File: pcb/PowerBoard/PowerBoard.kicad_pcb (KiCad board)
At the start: 2 copper layers, 9 parts, among them P1 Motor battery, P2 CONN_01X06, P3 Arduino battery, SW1 OnOffDoubleSwitch

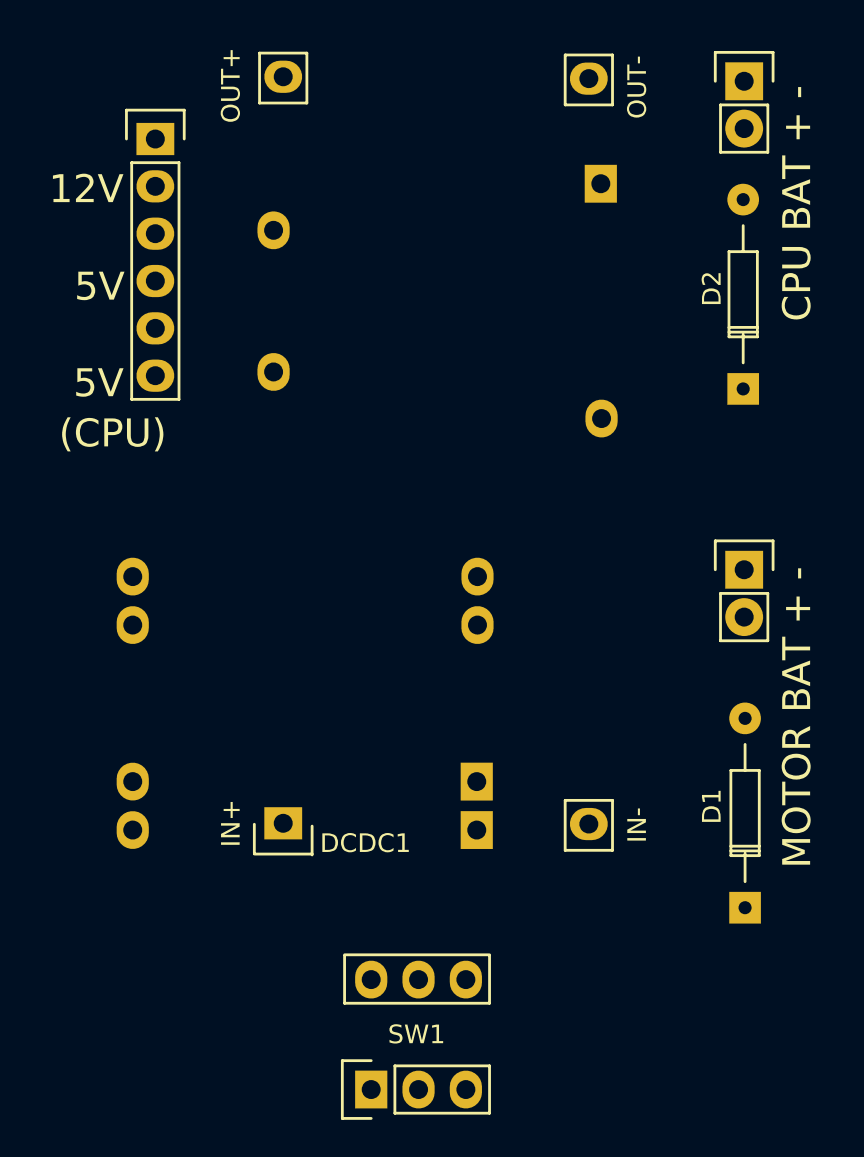
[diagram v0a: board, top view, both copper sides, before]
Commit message: power board ready
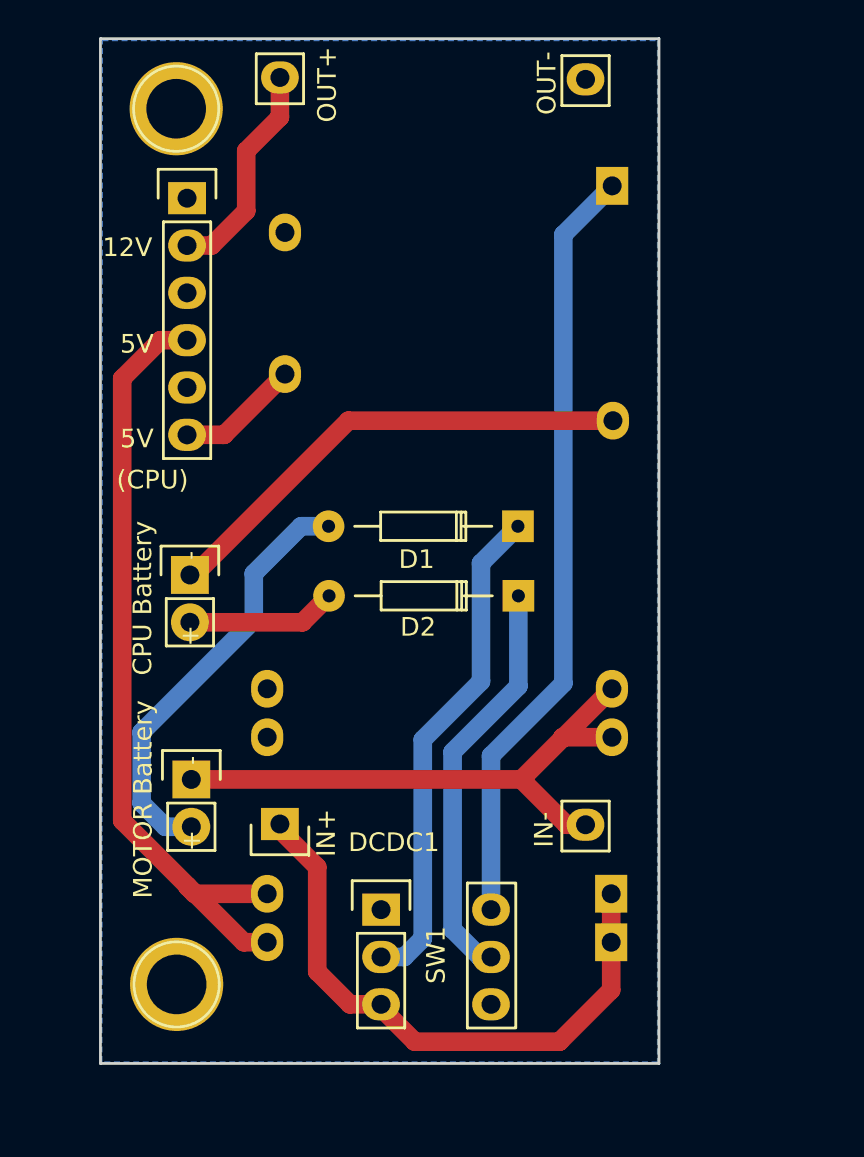
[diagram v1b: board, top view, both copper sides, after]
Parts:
- added REF**: 1pin, Connect:1pin, F.Cu at (130.5, 128.4)
- added REF**: 1pin, Connect:1pin, F.Cu at (130.5, 81.4)
- moved P3 39.8 mm to (131.2, 106.5)
- moved P1 31.7 mm to (131.3, 117.4)
- moved D1 23.8 mm to (148.8, 103.8), turned to 180 degrees
- moved D2 16.4 mm to (148.8, 107.6), turned to 180 degrees
- moved DCDC2 9.40 mm to (145.9, 119.7)
- moved SW1 7.40 mm to (144.4, 124.5), turned to 0 degrees
- moved P2 3.60 mm to (131.0, 86.2)
- moved DCDC3 0.62 mm to (133.5, 91.9)
- moved DCDC1 0.18 mm to (144.2, 99.4)
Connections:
- net Net-(DCDC1-Pad4) renamed GND
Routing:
- net Net-(DCDC2-Pad3): track 0.00 -> 43.0 mm
- net Net-(DCDC3-Pad1): track 0.00 -> 41.5 mm
- net Net-(DCDC1-Pad1): track 0.00 -> 32.5 mm
- net Net-(DCDC1-Pad2): track 0.00 -> 31.8 mm
- net Net-(D1-Pad1): track 0.00 -> 26.9 mm
- net Net-(DCDC3-Pad2): track 0.00 -> 26.1 mm
- net Net-(D1-Pad2): track 0.00 -> 23.1 mm
- net Net-(D2-Pad1): track 0.00 -> 22.0 mm
- net Net-(DCDC1-Pad3): track 0.00 -> 11.9 mm
- net Net-(D2-Pad2): track 0.00 -> 8.06 mm
- net Net-(DCDC3-Pad3): track 0.00 -> 6.60 mm
- added copper zone on B.Cu, net GND
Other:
- board outline added: 30 x 55 mm
- net class power added: clearance 0.5, trace_width 1, via_dia 1.5, via_drill 0.8
- board text added: "+ -"
- board text added: "CPU Battery"
- board text added: "MOTOR Battery"
- board text removed: "CPU BAT + -"
- board text removed: "MOTOR BAT + -"
